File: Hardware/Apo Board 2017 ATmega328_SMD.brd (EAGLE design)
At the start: 85.1 x 52.7 mm, 33 parts, among them Q1 RESONATORSMD, U1 LED-TRICOLOR-5050-IC, U10 LED-TRICOLOR-5050-IC, U11 LED-TRICOLOR-5050-IC, U13 ATMEGA328, U3 LED-TRICOLOR-5050-IC, U4 LED-TRICOLOR-5050-IC, U5 LED-TRICOLOR-5050-IC, U6 LED-TRICOLOR-5050-IC, U7 LED-TRICOLOR-5050-IC, U8 LED-TRICOLOR-5050-IC, U9 LED-TRICOLOR-5050-IC

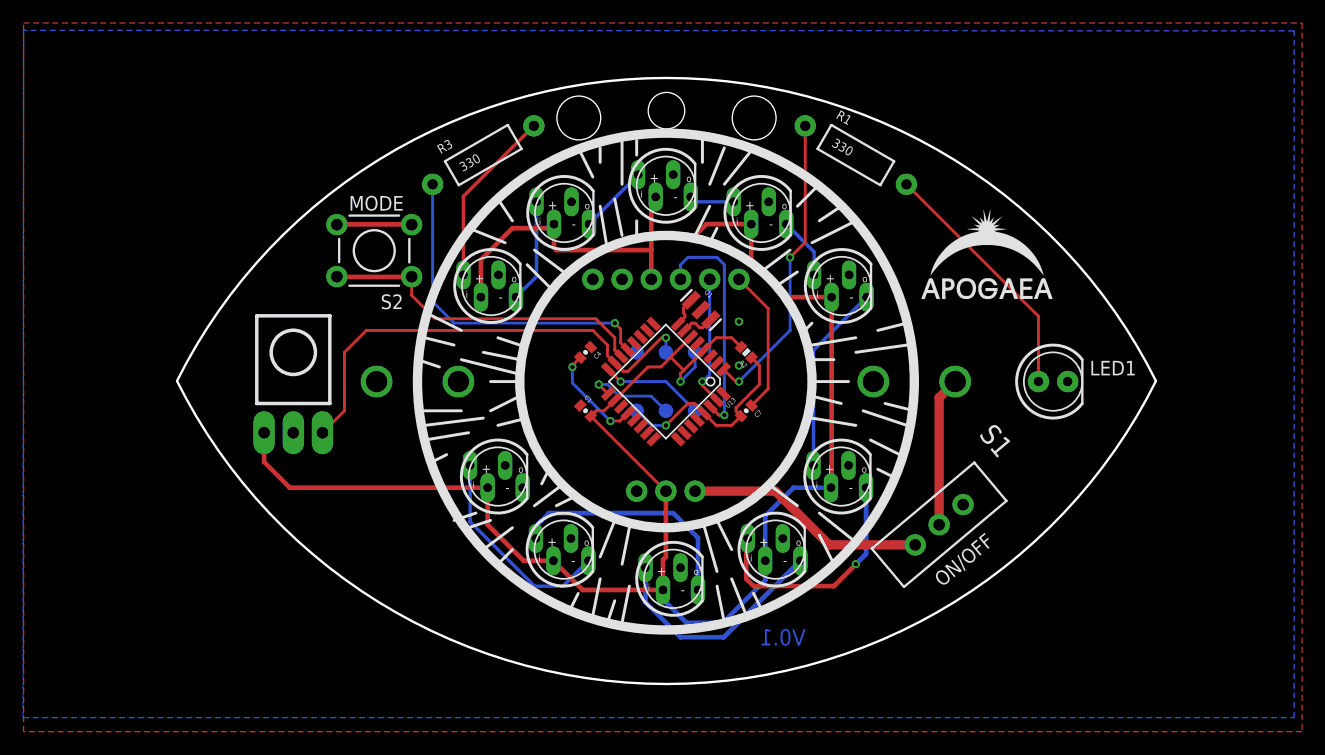
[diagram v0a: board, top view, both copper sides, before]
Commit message: Power Tests
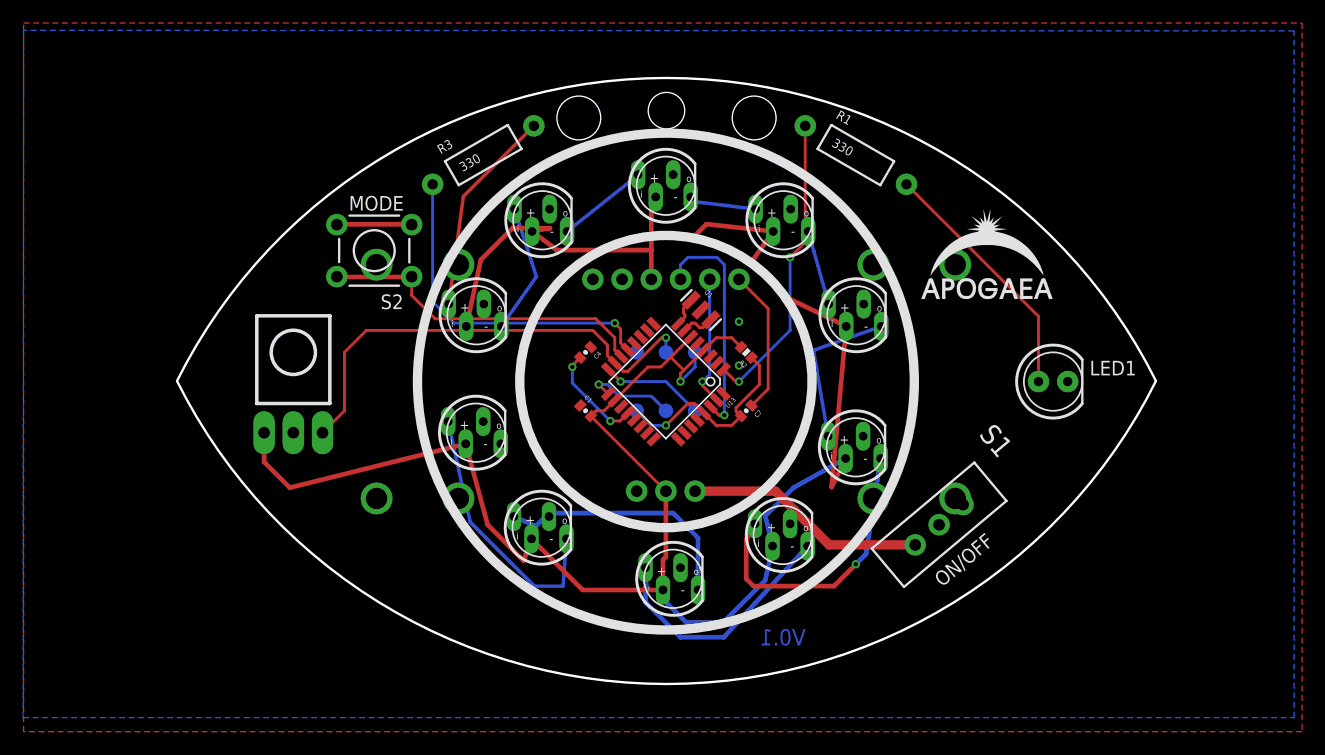
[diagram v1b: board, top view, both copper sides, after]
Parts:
- added BAT2: AA, SparkFun:BATTERY-AA-KIT
- moved BAT1 10.2 mm to (0.00, -10.2)
- moved U8 4.26 mm to (-16.5, -4.45)
- moved U11 2.84 mm to (16.5, -5.71)
- moved U4 2.84 mm to (16.6, 5.77)
- moved U7 2.84 mm to (-16.5, 5.77)
- moved U1 2.69 mm to (-10.8, -12.7)
- moved U3 2.01 mm to (10.2, 14.0)
- moved U6 2.01 mm to (-10.7, 14.0)
- moved U10 1.42 mm to (10.2, -13.3)
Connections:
- new net N$10: BAT1.PWR@1, BAT2.GND@1
- net N$7: now also BAT2.PWR@1; no longer BAT1.PWR@1
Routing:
- net +5V: track 175.9 -> 190.8 mm
- net N$7: track 13.0 -> 0.00 mm
- net N$14: track 18.4 -> 23.4 mm
- net N$9: track 21.2 -> 25.2 mm
- net DOUT_DIN: track 16.5 -> 13.8 mm
- net LED_PIN: track 15.5 -> 18.1 mm
- net N$1: track 9.02 -> 11.5 mm
- net N$5: track 3.91 -> 5.85 mm
- net N$2: track 6.07 -> 7.91 mm
- net N$11: track 20.5 -> 21.8 mm
- net N$6: track 5.41 -> 6.56 mm
- net N$13: track 21.1 -> 22.1 mm
